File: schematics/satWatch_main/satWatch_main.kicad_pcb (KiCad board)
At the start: 4 copper layers, 45.2 x 28 mm, 55 parts, among them J1 POGO_03x14, J2 Pogo_02x03_UARTPROG, Q1 DMP1045U, Q2 BSS138, Q3 BSS138, SW1 B3U-1000P, SW2 B3U-1000P, SW3 EVQ-P7C01P, SW4 EVQ-P7C01P, SW5 EVQ-P7C01P, U1 PAM2401SCADJ, U2 MIC5365-1.8YC5, U3 ESP32-S3-MINI-1, U4 MAX30101EFD_T, U5 BNO085, U6 DS3231MZ, Y1 32.768Hz

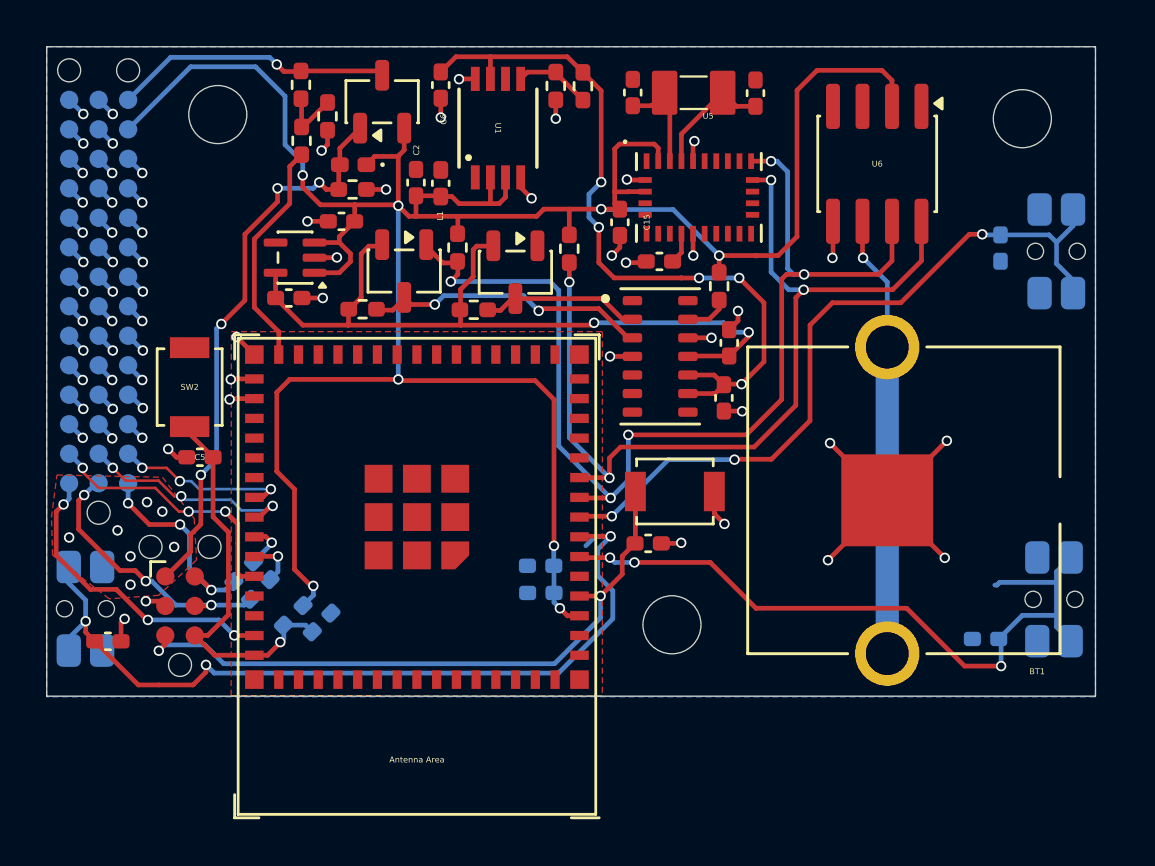
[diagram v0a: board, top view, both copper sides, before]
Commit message: V0.65
mainboard progress backup
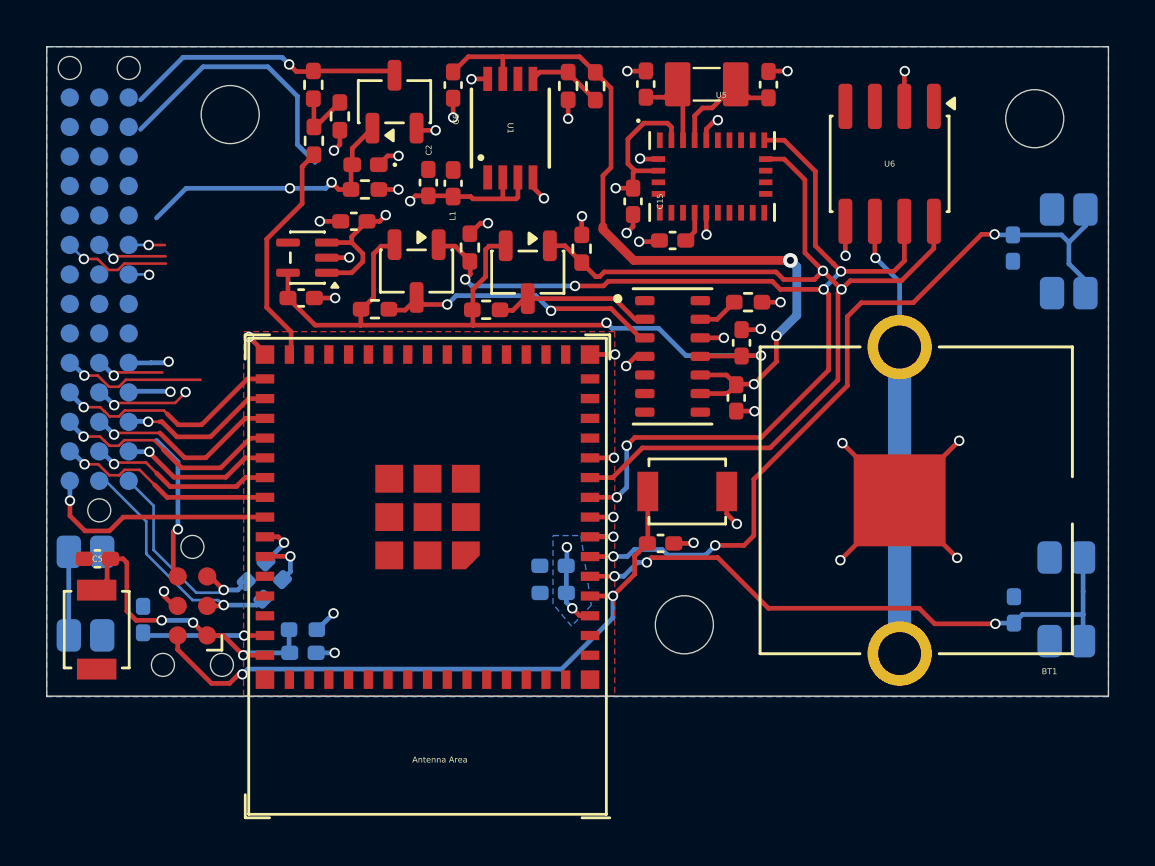
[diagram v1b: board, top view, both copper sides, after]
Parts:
- C12: moved to B.Cu
- SW3, SW4, SW5: value EVQ-P7C01P -> EVQ-P7A01P; footprint Button_Switch_SMD:SW_SPST_EVQP7C -> Button_Switch_SMD:SW_SPST_EVQP7A
- moved SW2 11.2 mm to (129.2, 101.3), turned to 90 degrees
- moved C5 6.21 mm to (129.2, 98.2)
- moved C12 1.78 mm to (131.2, 100.9), turned to 90 degrees
- moved C11 1.75 mm to (168.7, 100.5), turned to 90 degrees
- moved C7 1.54 mm to (138.0, 102.3), turned to 0 degrees
- moved R12 1.42 mm to (157.2, 87.2), turned to 0 degrees
- moved U5 1.07 mm to (155.7, 81.8)
- moved C15 1.07 mm to (152.2, 82.9)
- moved C16 1.07 mm to (154.0, 84.5)
- moved R5 0.74 mm to (138.0, 101.3), turned to 180 degrees
- moved C17 0.67 mm to (158.1, 77.8)
- moved C18 0.67 mm to (152.8, 77.8)
- moved Y1 0.67 mm to (155.4, 77.8)
- moved SW4 0.65 mm to (128.7, 99.8)
- moved BT1 0.53 mm to (163.7, 95.7)
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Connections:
- C11 pad 1: /GPIO2/BUTTON1 -> /GPIO1/BUTTON1
- C12 pad 1: /GPIO3/BUTTON2 -> /GPIO46/BUTTON2
- C14 pad 1: /GPIO4/BUTTON3 -> /GPIO2/BUTTON3
- J1 pad 11: /GPIO35 -> /GPIO4
- J1 pad 12: /GPIO38 -> /GPIO36
- J1 pad 13: /GPIO41 -> /GPIO39
- J1 pad 25: /GPIO36 -> /GPIO3
- J1 pad 26: /GPIO39 -> /GPIO37
- J1 pad 27: /GPIO42 -> /GPIO40
- J1 pad 38: unconnected-(J1-Pin_38-Pad38) -> /GPIO2
- J1 pad 39: /GPIO37 -> /GPIO35
- J1 pad 40: /GPIO40 -> /GPIO38
- J1 pad 41: /GPIO45 -> /GPIO41
- J1 pad 42: /GPIO46 -> /GPIO42
- J2 pad 1: VIN_3V3 -> /EN/CHIP_PU
- J2 pad 2: GND -> /U0RXD
- J2 pad 3: /GPIO0/BOOT -> /U0TXD
- J2 pad 4: /EN/CHIP_PU -> VIN_3V3
- J2 pad 5: /U0RXD -> GND
- J2 pad 6: /U0TXD -> /GPIO0/BOOT
- SW3 pad 2: /GPIO2/BUTTON1 -> /GPIO1/BUTTON1
- SW4 pad 2: /GPIO3/BUTTON2 -> /GPIO46/BUTTON2
- SW5 pad 2: /GPIO4/BUTTON3 -> /GPIO2/BUTTON3
- U3 pad 44: /GPIO46 -> /GPIO46/BUTTON2
- U3 pad 5: /GPIO1 -> /GPIO1/BUTTON1
- U3 pad 6: /GPIO2/BUTTON1 -> /GPIO2/BUTTON3
- U3 pad 7: /GPIO3/BUTTON2 -> /GPIO3
- U3 pad 8: /GPIO4/BUTTON3 -> /GPIO4
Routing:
- net 3V3: track 114.9 -> 41.6 mm, vias 8 -> 12
- net /GPIO3/BUTTON2: track 36.9 -> 0.00 mm, vias 3 -> 0
- net /GPIO2/BUTTON3: track 0.00 -> 34.1 mm, vias 0 -> 3
- net /GPIO4/BUTTON3: track 32.3 -> 0.00 mm, vias 3 -> 0
- net /GPIO2/BUTTON1: track 31.0 -> 0.00 mm, vias 3 -> 0
- net /GPIO1/BUTTON1: track 0.00 -> 26.5 mm, vias 0 -> 3
- net /GPIO46: track 13.3 -> 0.00 mm, vias 3 -> 0
- net /GPIO45: track 11.5 -> 0.00 mm, vias 3 -> 0
- net /GPIO38: track 0.85 -> 9.94 mm
- net /GPIO46/BUTTON2: track 0.00 -> 8.44 mm, vias 0 -> 1
- net /GPIO35: track 1.87 -> 9.99 mm, vias 2 -> 1
- net /GPIO37: track 0.86 -> 8.54 mm
- net /GPIO40: track 0.79 -> 7.98 mm
- net /GPIO3: track 0.00 -> 6.46 mm, vias 0 -> 3
- net /GPIO2: track 0.00 -> 6.19 mm, vias 0 -> 1
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- added copper zone on B.Cu, net (none)
- added copper zone on In2.Cu, net 3V3
- added copper zone on In1.Cu, net GND
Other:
- board size 45.2 x 28 mm -> 45.7 x 28 mm
